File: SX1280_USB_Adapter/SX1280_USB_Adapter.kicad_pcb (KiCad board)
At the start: 2 copper layers, 45 x 19.6 mm, 27 parts, among them J1 USB_A_PLUG, U1 AMS1117-3.3, U2 CH341a, U3 SX1280, Y1 Crystal_GND24

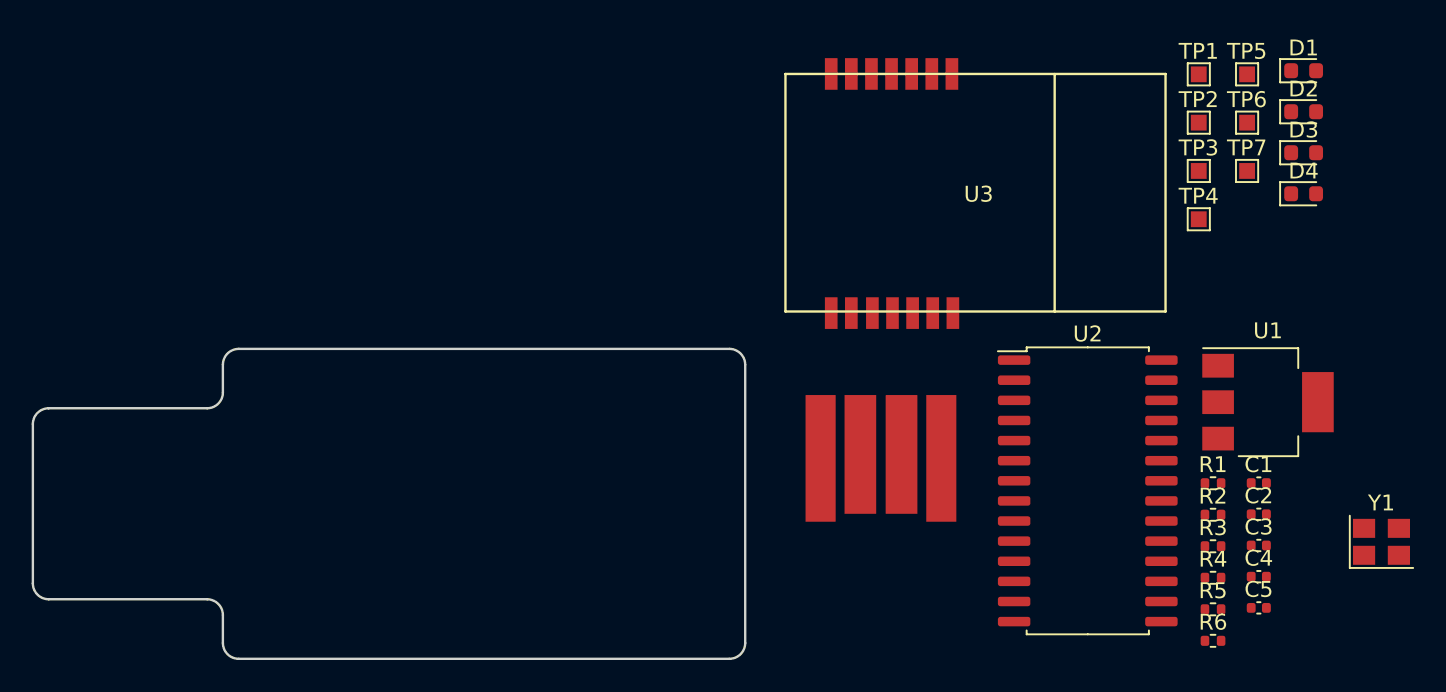
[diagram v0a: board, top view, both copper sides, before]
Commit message: update layout
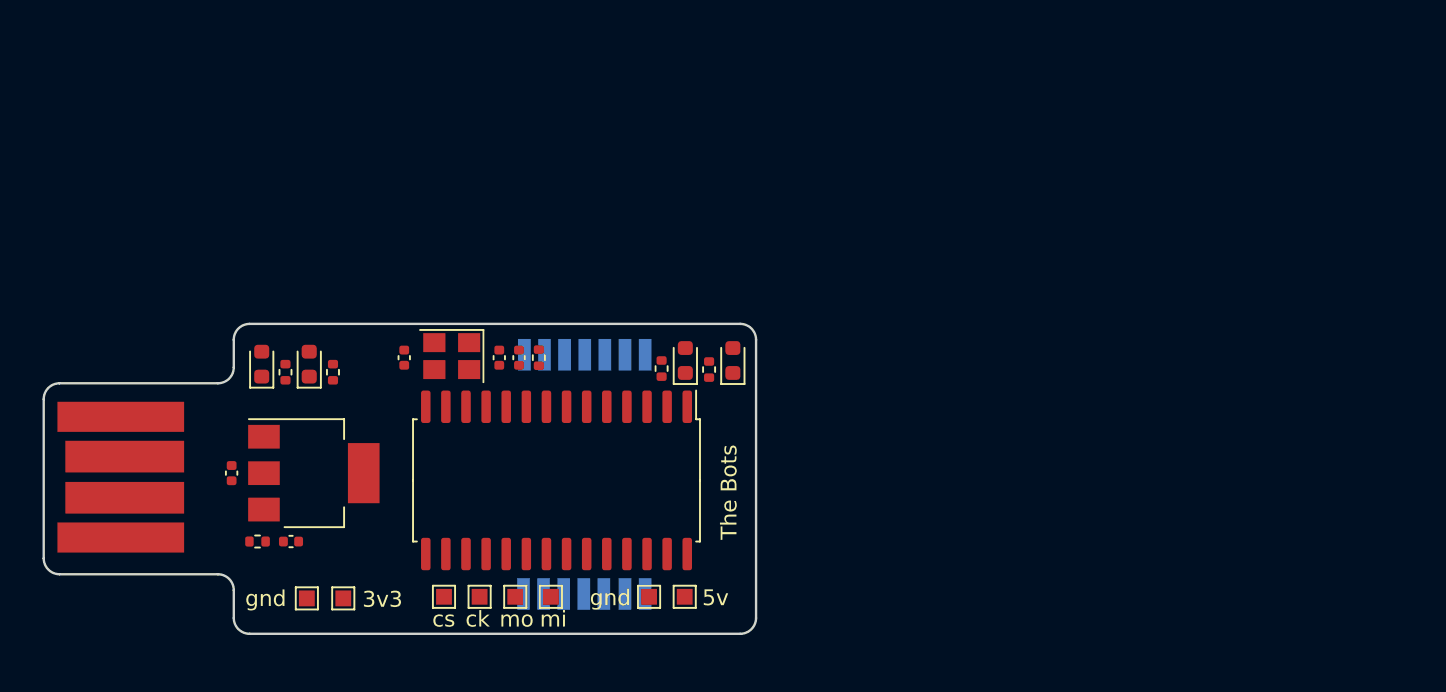
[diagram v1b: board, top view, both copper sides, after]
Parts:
- added TP8: TestPoint, TestPoint:TestPoint_Pad_1.0x1.0mm, F.Cu at (113.3, 121.7)
- U3: moved to B.Cu
- moved D1 68.4 mm to (110.5, 106.9), turned to 90 degrees
- moved C2 64.9 mm to (108.6, 113.8), turned to -90 degrees
- moved D4 63.7 mm to (113.5, 106.9), turned to 90 degrees
- moved TP2 61.8 mm to (115.7, 121.7)
- moved C5 61.3 mm to (112.3, 118.1)
- moved R1 60.4 mm to (110.2, 118.1), turned to 180 degrees
- moved U1 60.4 mm to (113.8, 113.8)
- moved Y1 59.9 mm to (122.5, 106.4), turned to 180 degrees
- moved R2 59.3 mm to (112.0, 107.4), turned to 90 degrees
- moved TP6 58.9 mm to (122.0, 121.6)
- moved TP5 56.8 mm to (126.5, 121.6)
- moved R3 56.6 mm to (115.0, 107.4), turned to 90 degrees
- moved C4 55.7 mm to (119.5, 106.5), turned to -90 degrees
- moved TP7 55.4 mm to (124.3, 121.6)
- moved J1 53.0 mm to (96.7, 114.0), turned to -90 degrees
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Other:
- board text added: "3v3"
- board text added: "5v"
- board text added: "The Bots"
- board text added: "ck"
- board text added: "cs"
- board text added: "gnd"
- board text added: "mi"
- board text added: "mo"
